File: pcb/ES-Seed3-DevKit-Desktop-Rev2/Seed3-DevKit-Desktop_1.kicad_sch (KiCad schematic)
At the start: 56 parts, among them J7 USB4110GFA, U12 CD4051B, U14 USBLC6-2SC6, U2 MCP6002-xSN, U4 4021, U5 4021, U6 MCP6002-xSN, U9 MCP6002-xSN

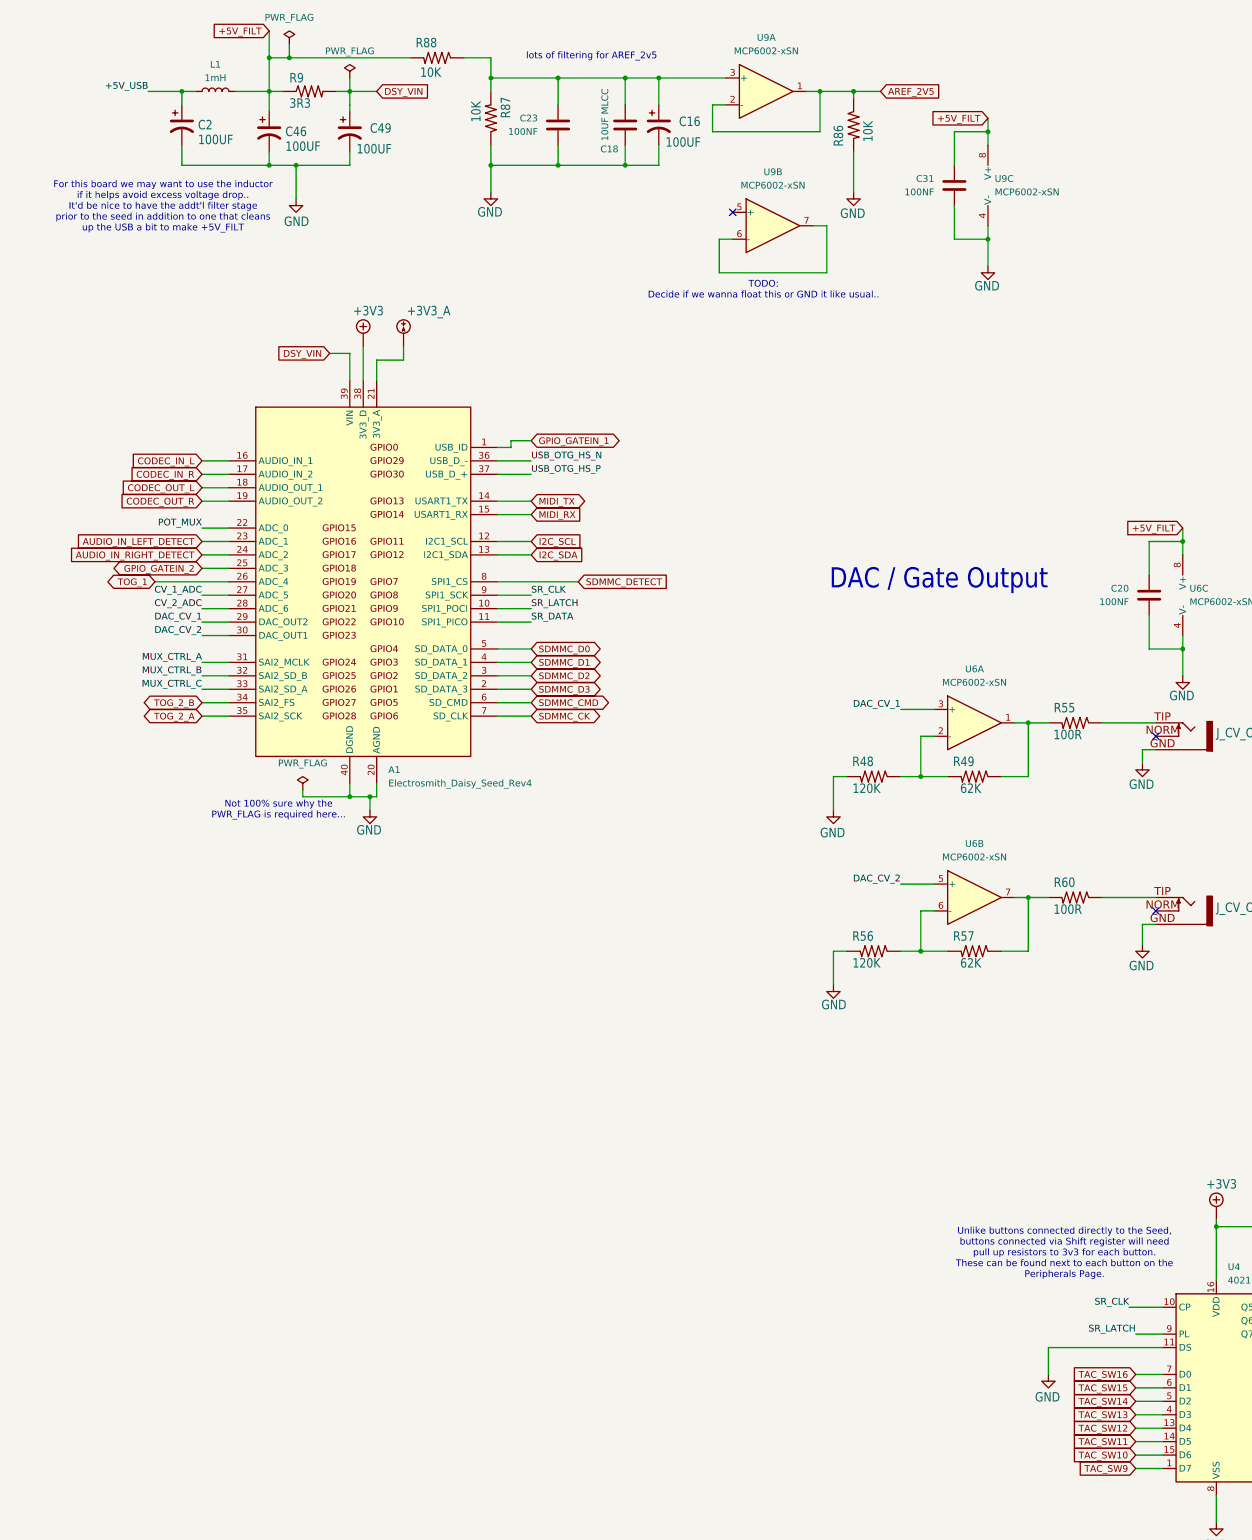
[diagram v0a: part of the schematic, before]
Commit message: starting to add the boost circuit changes now that the easy stuff is done.
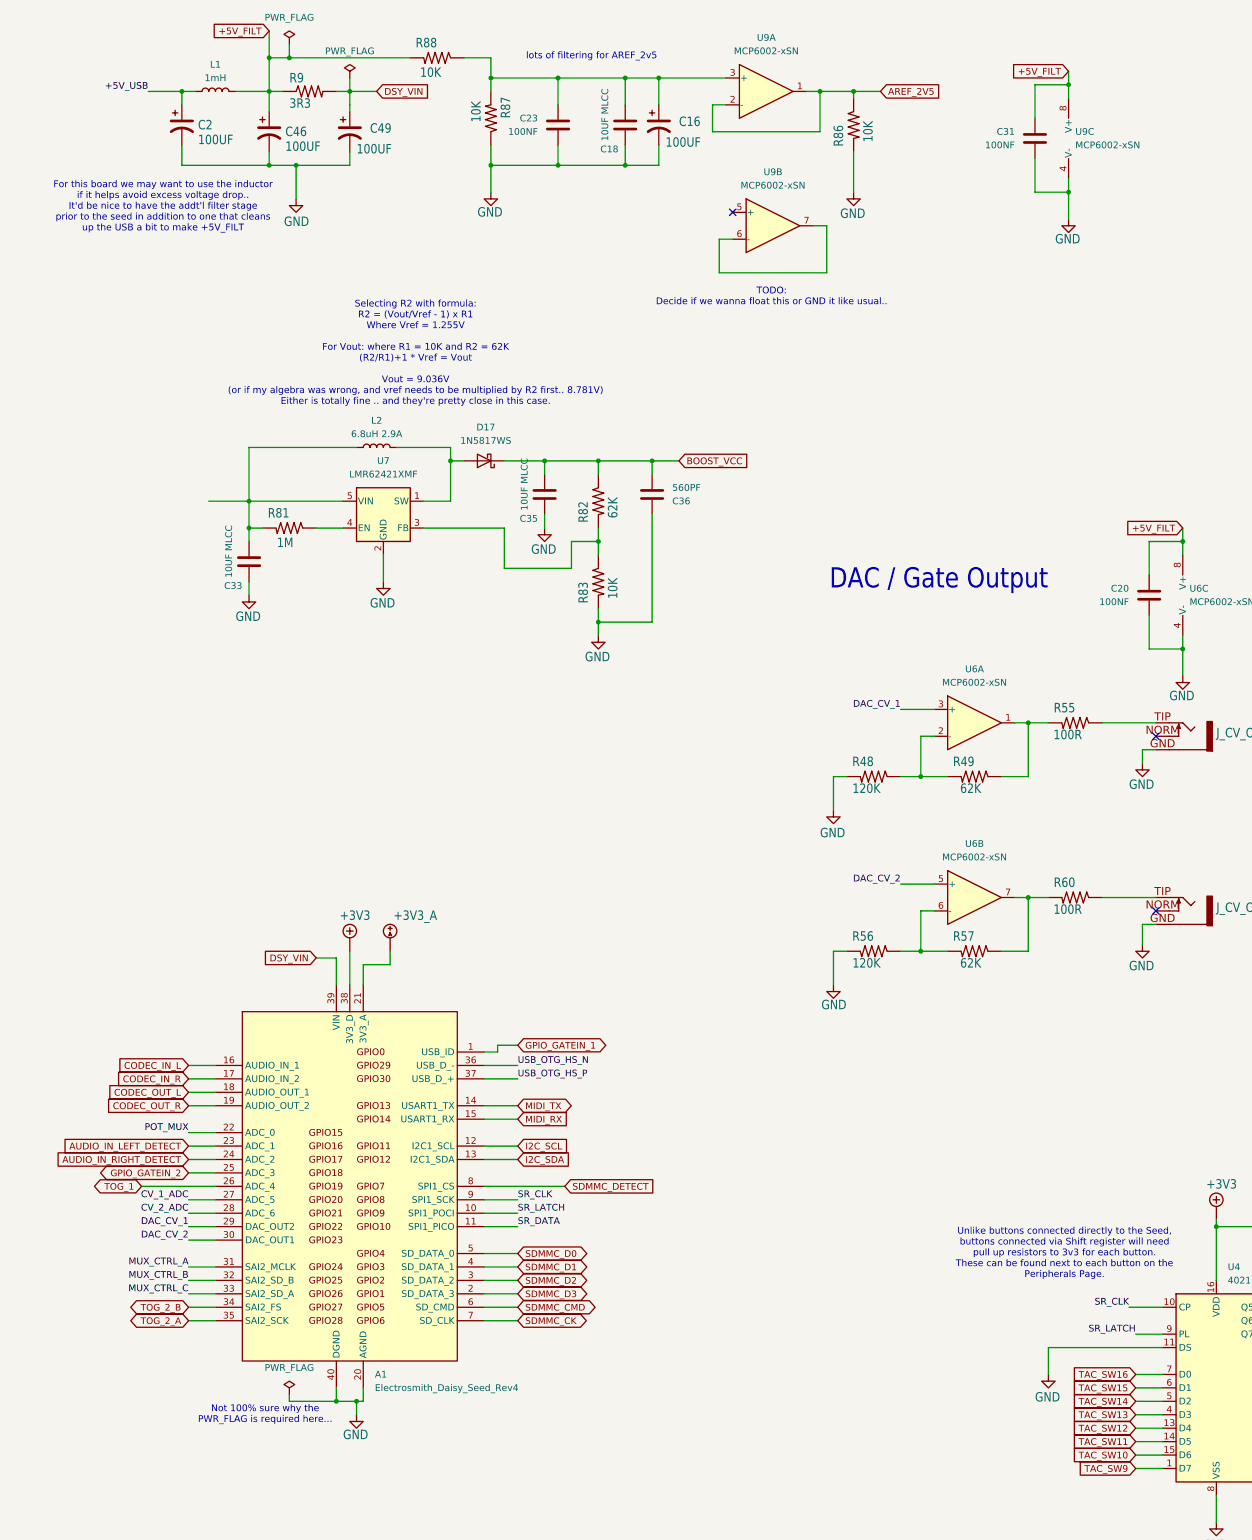
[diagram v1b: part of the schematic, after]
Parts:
- added C33, C35: 10UF MLCC, Capacitor_SMD:C_0805_2012Metric, symbol Device:C
- added C36: 560PF, Capacitor_SMD:C_0603_1608Metric, symbol Device:C
- added D17: 1N5817WS, Diode_SMD:D_SOD-323F, symbol Device:D_Schottky
- added L2: 6.8uH 2.9A, symbol Device:L
- added R81: 1M, Resistor_SMD:R_0603_1608Metric, symbol Seed3-Pedal-DevKit-Converted-eagle-import:Electrosmith-Passives_R-US_R0603
- added R82: 62K, Resistor_SMD:R_0603_1608Metric, symbol Seed3-Pedal-DevKit-Converted-eagle-import:Electrosmith-Passives_R-US_R0603
- added R83: 10K, Resistor_SMD:R_0603_1608Metric, symbol Seed3-Pedal-DevKit-Converted-eagle-import:Electrosmith-Passives_R-US_R0603
- added U7: LMR62421XMF, Package_TO_SOT_SMD:SOT-23-5, symbol Regulator_Switching:LMR62421XMF
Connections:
- net GND: now also C33.2, C35.2, C36.1, R83.2, U7.2 (GND)
- new net: D17.2 (A), L2.2, U7.1 (SW)
- new net: R82.2, R83.1, U7.3 (FB)
- new net: R81.1, U7.4 (EN)
- new net: C33.1, L2.1, R81.2, U7.5 (VIN)
- new net BOOST_VCC: C35.1, C36.2, D17.1 (K), R82.1
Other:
- note added: "Selecting R2 with formula: R2 = (Vout/Vref - 1) x R1 Where Vref = 1.255V For Vout: where R1 = 10K and R2 = 62K (R2/R1)+1 * Vref = Vout Vout = 9.036V (or if my algebra was wrong, and vref needs to be multiplied by R2 first.. 8.781V) Either is totally fine .. and they're pretty close in this case."
- moved on the sheet: A1, C31, U9C

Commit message: layout and routing for changes -- need to review, and make mats.
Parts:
- removed L1: 1mH, shnsly:L_SDR0805, symbol Device:L
- added C37, C38, C39, C41: 100UF, Capacitor_SMD:CP_Elec_6.3x7.7, symbol Device:C_Polarized_US
- added C40: 100NF, Capacitor_SMD:C_0603_1608Metric, symbol Device:C
- added D18, D19, D20, D25: 1N5817WS, Diode_SMD:D_SOD-323F, symbol Device:D_Schottky
- added R84: 0R, Resistor_SMD:R_0603_1608Metric, symbol Seed3-Pedal-DevKit-Converted-eagle-import:Electrosmith-Passives_R-US_R0603
- added R95, R97, R98, R99: 3R3, Resistor_SMD:R_1206_3216Metric, symbol Seed3-Pedal-DevKit-Converted-eagle-import:Electrosmith-Passives_R-US_R0603
- added U10: LD1117S50TR_SOT223, Package_TO_SOT_SMD:SOT-223-3_TabPin2, symbol Regulator_Linear:LD1117S50TR_SOT223
- L2: footprint (none) -> Inductor_SMD:L_TDK_VLS6045EX_VLS6045AF
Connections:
- net +3V3: now also D18.1 (K), D19.1 (K)
- net +5V_FILT: now also C41.1, R99.2; no longer C46.1, R88.2, R9.1
- net +5V_USB: now also R84.2; no longer C2.1
- net AUDIO_IN_LEFT_DETECT: now also D18.2 (A), D25.1 (K)
- net AUDIO_IN_RIGHT_DETECT: now also D19.2 (A), D20.1 (K)
- net BOOST_VCC: now also C37.1, R95.1, R97.1
- net GND: now also C37.2, C38.2, C39.2, C40.2, C41.2, D20.2 (A), D25.2 (A), U10.1 (GND); no longer C36.1
- net at R82.2, R83.1, U7.3 (FB): now also C36.1
- net at C33.1, L2.1, R81.2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: now also R84.1
- net AREF_2V5 renamed AREF_AUDIO_BIAS
- new net: C38.1, R97.2, R98.1
- new net: C46.1, R9.1, R95.2
- new net: C2.1, R99.1, U10.2 (VO)
- new net +9V_A: C39.1, C40.1, R88.2, R98.2, U10.3 (VI)
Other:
- note added: "Approx. 4.3V"
- note added: "At the moment, the +5V is powering: - Headphone Amp - DAC output op-amp - Reference voltage for CV inputs - 6002 buffer for AREF_AUDIO_BIAS We can remove this, and simplify slightly if we: - Power Headphone Amp from +3v3_A - Change DAC output op-amp to a rail-to-rail opamp that supports higher voltage (i.e. OPA1652) - Power DAC output op-amp from +9V_A - Add LM4040 for +5V reference for CV inputs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"
- note added: "Jump Point In case of troubleshooting or for testing power via battery if we want"
- note added: "POWER"
- note added: "Selecting R2 with formula: R2 = (Vout/Vref - 1) x R1 Where Vref = 1.255V For Vout: where R1 = 10K and R2 = 62K (R2/R1)+1 * Vref = Vout Vout = 9.036V (or if my algebra was wrong, it would be.. 8.781V) Either is totally fine .. and they're pretty close in this case."
- note added: "This will drop a fair amount of voltage Measured at ~7.86V on a similar circuit on Pedal Dev Kit Rev2"
- note added: "This will drop a fair amount of voltage Measured at ~8.6V on similar circuit on Pedal Dev Kit Rev2"
- note added: "lots of filtering for buffered midrail"
- note removed: "For this board we may want to use the inductor if it helps avoid excess voltage drop.. It'd be nice to have the addt'l filter stage prior to the seed in addition to one that cleans up the USB a bit to make +5V_FILT"
- note removed: "Selecting R2 with formula: R2 = (Vout/Vref - 1) x R1 Where Vref = 1.255V For Vout: where R1 = 10K and R2 = 62K (R2/R1)+1 * Vref = Vout Vout = 9.036V (or if my algebra was wrong, and vref needs to be multiplied by R2 first.. 8.781V) Either is totally fine .. and they're pretty close in this case."
- note removed: "lots of filtering for AREF_2v5"
- moved on the sheet: A1, C14, C15, C16, C18, C19, C20, C23, C31, C33, C35, C36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
